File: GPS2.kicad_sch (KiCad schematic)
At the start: 12 parts, among them J1 GPS_ANT_0, U1 MAX-M10S-00B

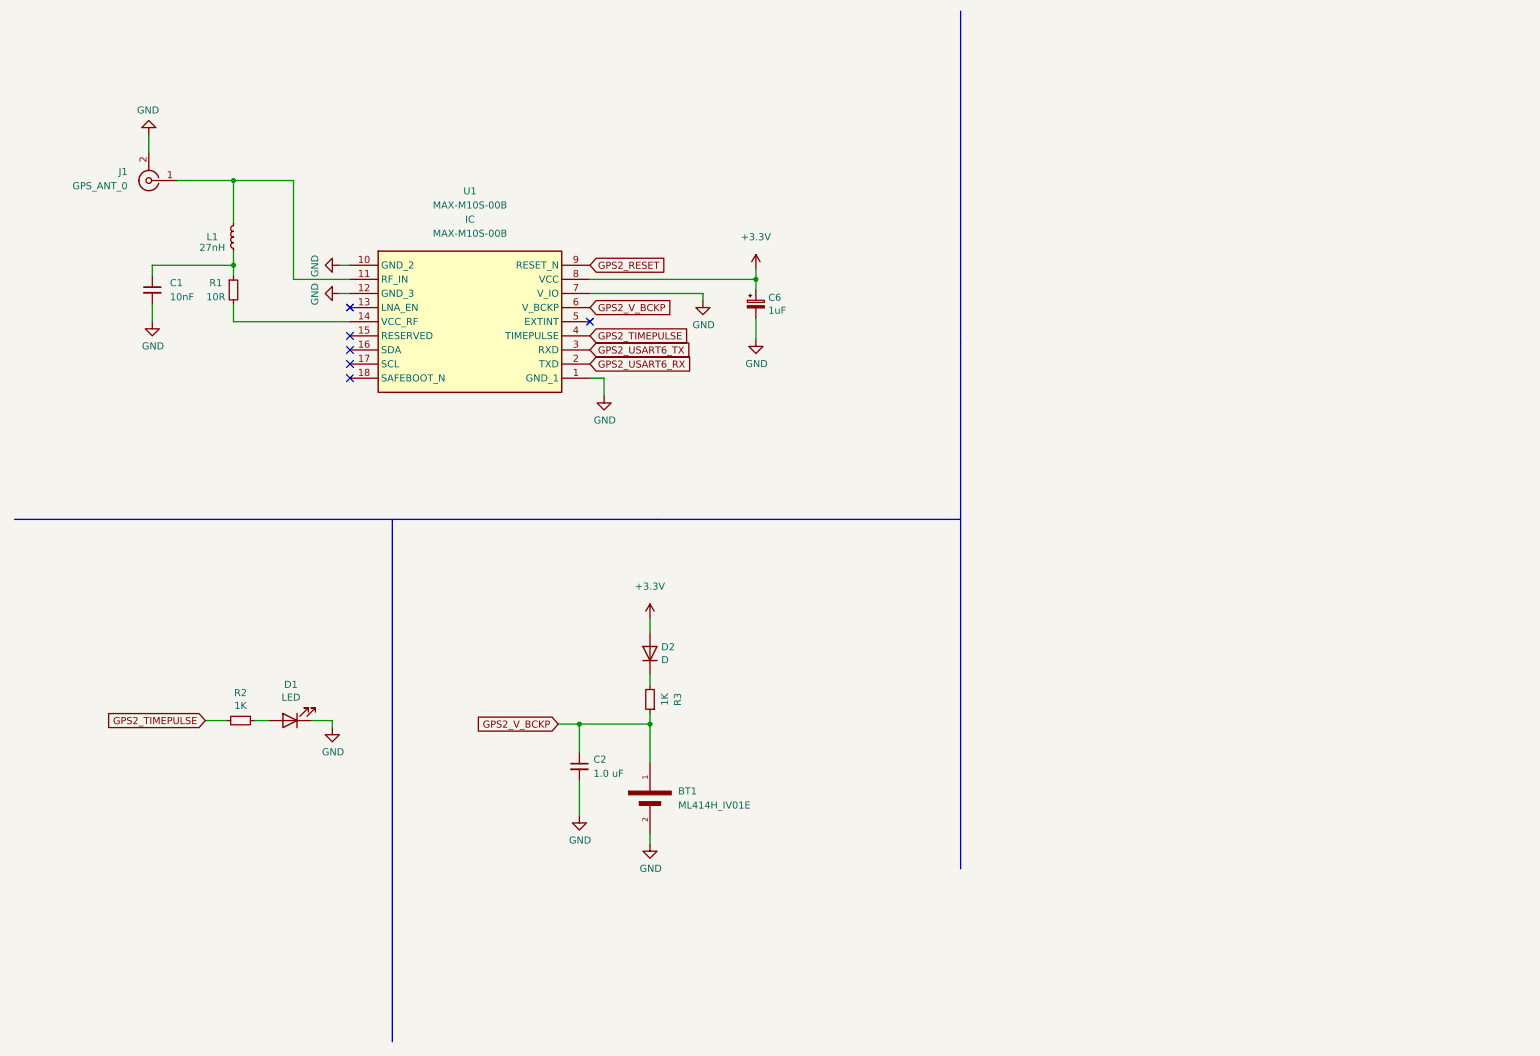
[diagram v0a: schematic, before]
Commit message: Last commit
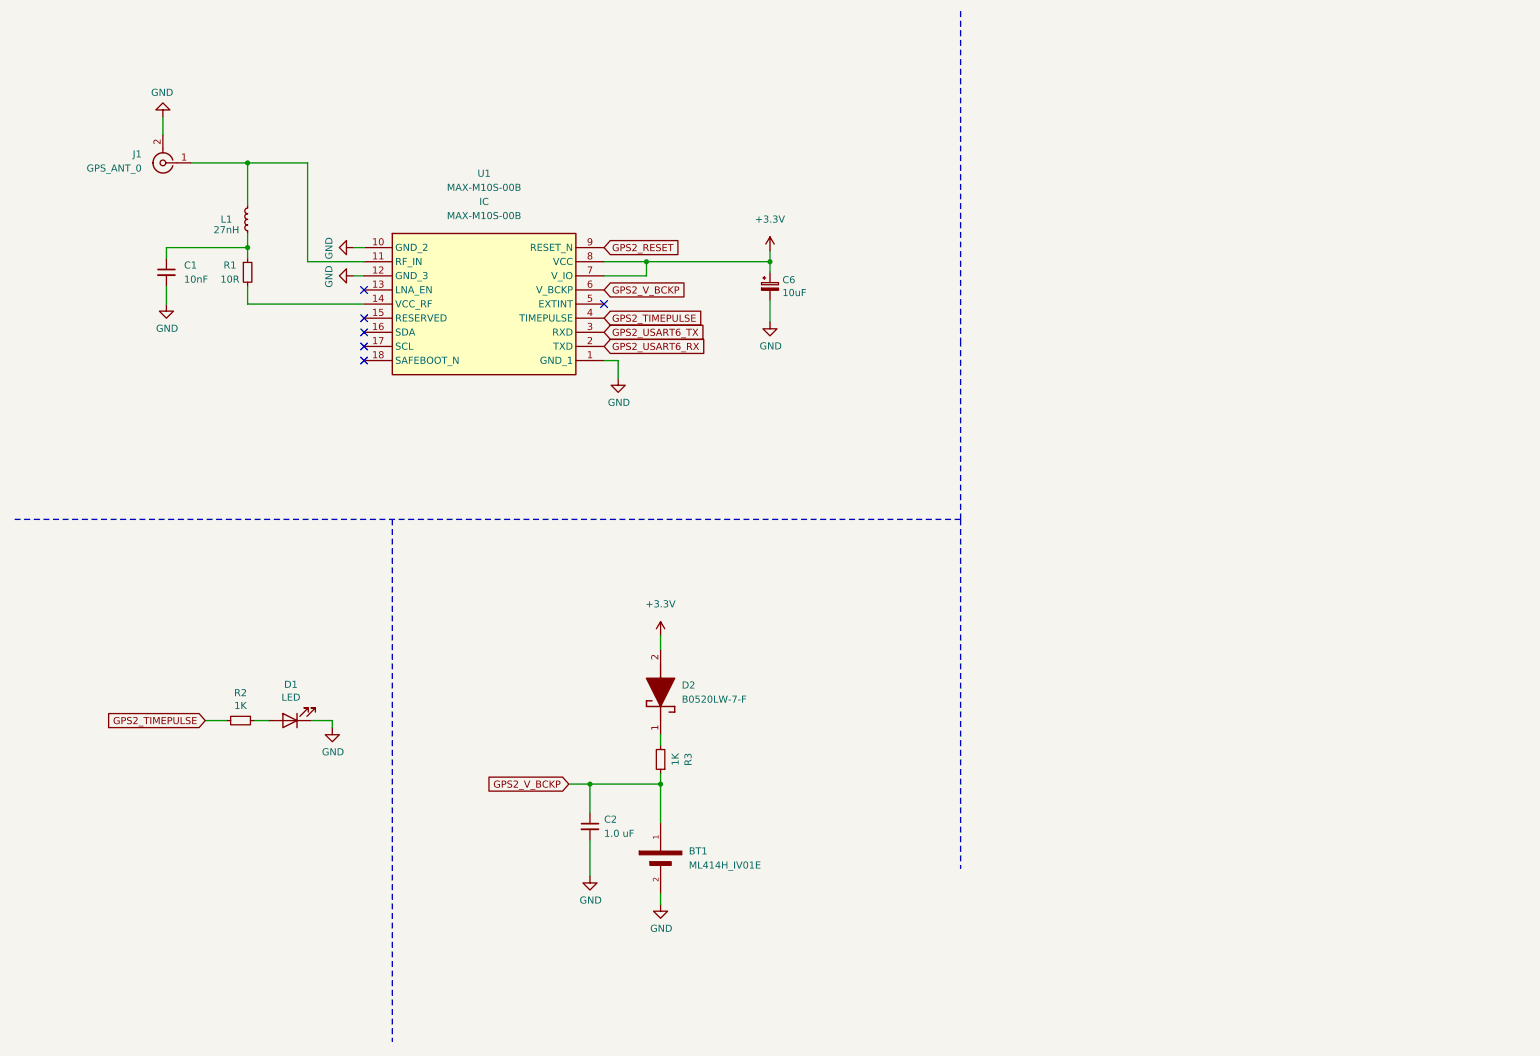
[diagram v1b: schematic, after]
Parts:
- removed D2: D, Diode_SMD:D_1206_3216Metric_Pad1.42x1.75mm_HandSolder, symbol Device:D
- added D2: B0520LW-7-F, B0520LW-7-F:SOD3716X145N, symbol B0520LW-7-F:B0520LW-7-F
- C6: value 1uF -> 10uF; footprint Capacitor_Tantalum_SMD:CP_EIA-3528-21_Kemet-B_Pad1.50x2.35mm_HandSolder -> Capacitor_SMD:C_1210_3225Metric
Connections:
- net +3.3V: now also U1.7 (V_IO), D2.2 (A)
- net GND: no longer U1.7 (V_IO)
- net at R3.2: now also D2.1 (K)
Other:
- moved on the sheet: BT1, C1, C2, C6, J1, L1, R1, R3, U1

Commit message: Second commit
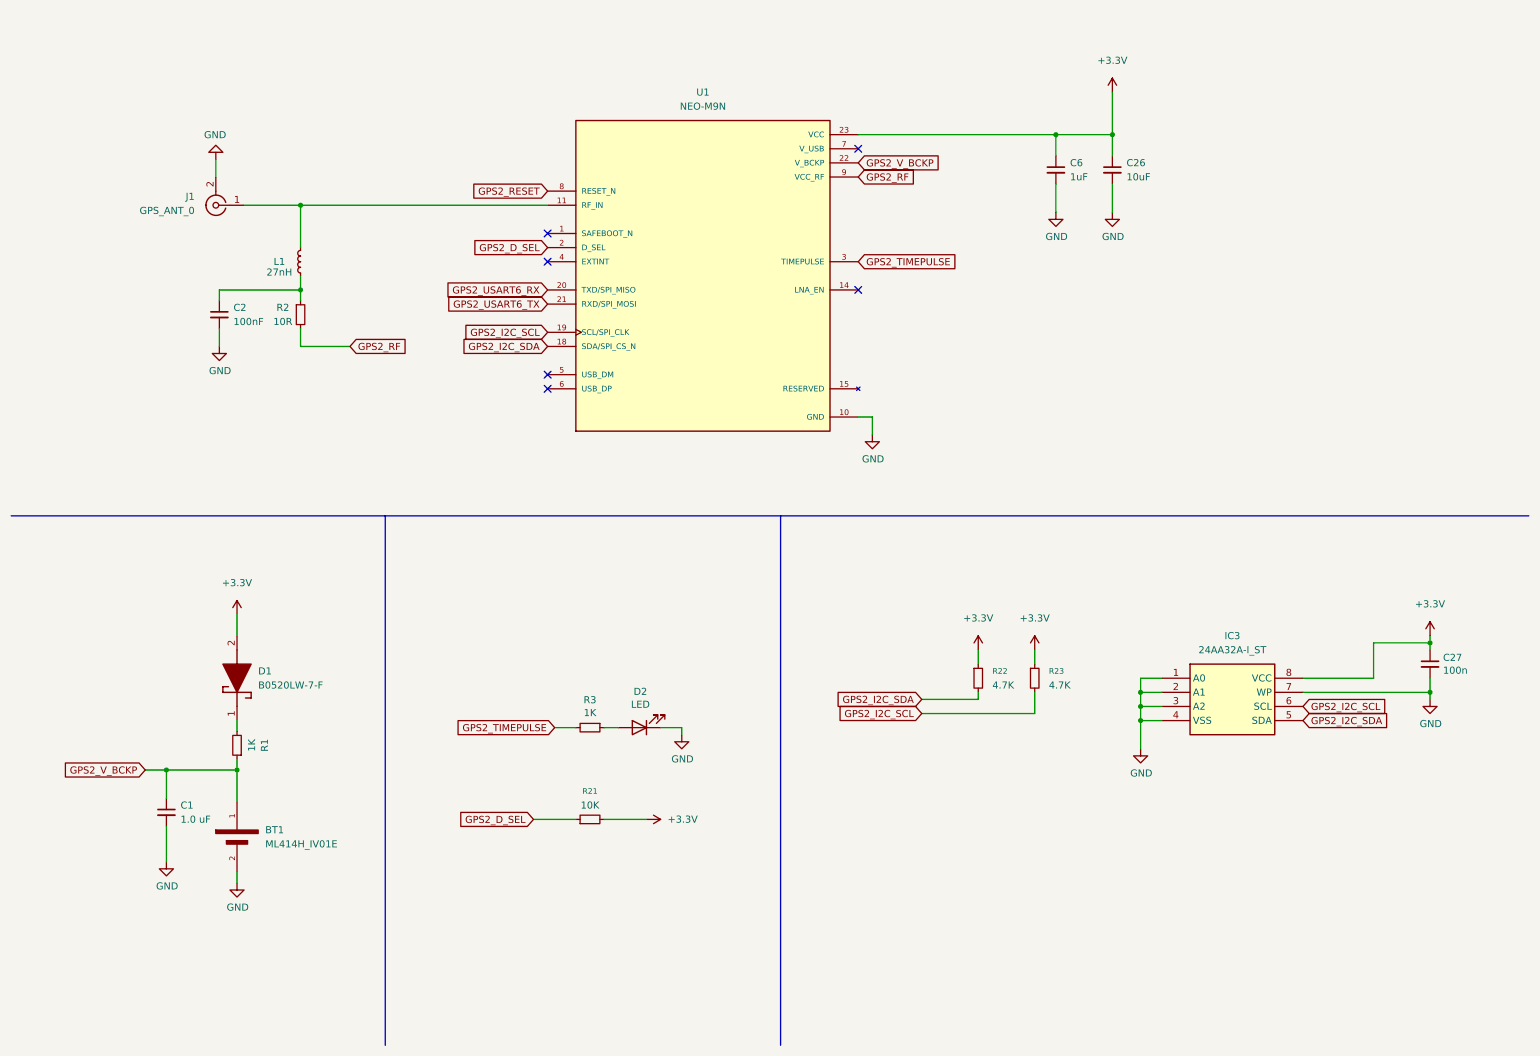
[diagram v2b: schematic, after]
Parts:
- removed C6: 10uF, Capacitor_SMD:C_1210_3225Metric, symbol Device:CP_Small
- removed D1: LED, LED_SMD:LED_0805_2012Metric_Pad1.15x1.40mm_HandSolder, symbol Device:LED
- removed D2: B0520LW-7-F, B0520LW-7-F:SOD3716X145N, symbol B0520LW-7-F:B0520LW-7-F
- removed U1: MAX-M10S-00B, MAX-M10S-00B:MAXM10S00B, symbol MAX-M10S-00B:MAX-M10S-00B
- added C26: 10uF, Capacitor_SMD:C_1210_3225Metric, symbol Device:C_Small
- added C27: 100n, Capacitor_SMD:C_0402_1005Metric, symbol Device:C_Small
- added C6: 1uF, Capacitor_SMD:C_1210_3225Metric, symbol Device:C_Small
- added D1: B0520LW-7-F, B0520LW-7-F:SOD3716X145N, symbol B0520LW-7-F:B0520LW-7-F
- added D2: LED, LED_SMD:LED_0805_2012Metric_Pad1.15x1.40mm_HandSolder, symbol Device:LED
- added IC3: 24AA32A-I_ST, 24AA32A-I_ST:SOP65P640X120-8N, symbol 24AA32A-I_ST:24AA32A-I_ST
- added R21: 10K, Resistor_SMD:R_0402_1005Metric, symbol Device:R_Small
- added R22, R23: 4.7K, Resistor_SMD:R_0402_1005Metric, symbol Device:R_Small
- added U1: NEO-M9N, NEO-M9N:XCVR_NEO-M9N, symbol NEO-M9N:NEO-M9N
- BT1: footprint ML414H_IV01E:SEIKO_ML414H_IV01E -> ML414H IV01E:SEIKO_ML414H_IV01E
- C1: value 10nF -> 1.0 uF; footprint Capacitor_SMD:C_0402_1005Metric -> Capacitor_SMD:C_0805_2012Metric
- C2: value 1.0 uF -> 100nF; footprint Capacitor_SMD:C_0805_2012Metric -> Capacitor_SMD:C_0402_1005Metric
- J1: footprint Connector_Coaxial:SMA_Samtec_SMA-J-P-X-ST-EM1_EdgeMount -> Connector_Coaxial:SMA_Samtec_SMA-J-P-H-ST-EM1_EdgeMount
- R1: value 10R -> 1K; footprint Resistor_SMD:R_0402_1005Metric -> Resistor_SMD:R_0805_2012Metric
- R2: value 1K -> 10R; footprint Resistor_SMD:R_0805_2012Metric -> Resistor_SMD:R_0402_1005Metric
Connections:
- net +3.3V: now also C26.1, C27.1, C6.1, D1.2 (A), IC3.8 (VCC), R21.2, R22.1, R23.1, U1.23 (VCC)
- net GND: now also C26.2, C27.2, C6.2, D2.1 (K), IC3.1 (A0), IC3.2 (A1), IC3.3 (A2), IC3.4 (VSS), IC3.7 (WP), U1.10 (GND), U1.12 (GND), U1.13 (GND), U1.24 (GND)
- net GPS2_RESET: now also U1.8 (RESET_N)
- net GPS2_TIMEPULSE: now also R3.2, U1.3 (TIMEPULSE); no longer R2.2
- net GPS2_USART6_RX: now also U1.20 (TXD/SPI_MISO)
- net GPS2_USART6_TX: now also U1.21 (RXD/SPI_MOSI)
- net GPS2_V_BCKP: now also C1.1, R1.1, U1.22 (V_BCKP); no longer C2.1, R3.1
- net at R2.1: now also C2.1, L1.1
- net at J1.1 (In), L1.2: now also U1.11 (RF_IN)
- net at R1.2: now also D1.1 (K)
- new net: D2.2 (A), R3.1
- new net: U1.15 (RESERVED), U1.16 (RESERVED), U1.17 (RESERVED)
- new net GPS2_D_SEL: R21.1, U1.2 (D_SEL)
- new net GPS2_I2C_SCL: IC3.6 (SCL), R23.2, U1.19 (SCL/SPI_CLK)
- new net GPS2_I2C_SDA: IC3.5 (SDA), R22.2, U1.18 (SDA/SPI_CS_N)
- new net GPS2_RF: R2.2, U1.9 (VCC_RF)
